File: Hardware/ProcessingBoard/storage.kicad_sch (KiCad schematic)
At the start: 21 parts, among them Q400 2N7002, U400 ADP163, U401 W25Q32JVZP

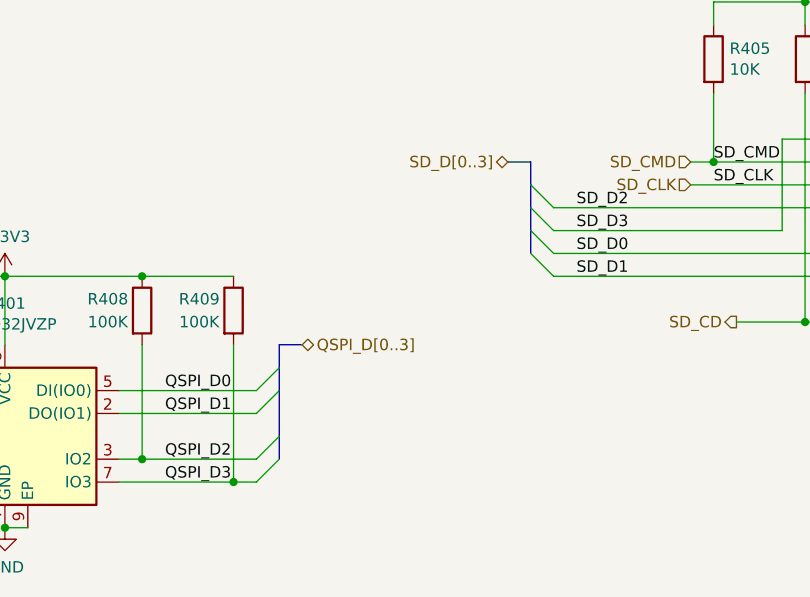
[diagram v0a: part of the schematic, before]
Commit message: Update License to match source code; test and fix USB, SEMC, and XIP on actual hardware
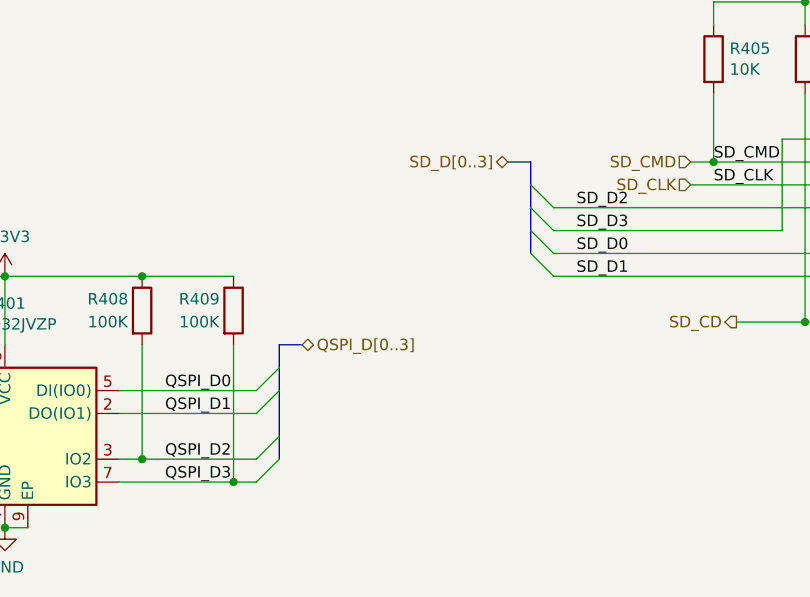
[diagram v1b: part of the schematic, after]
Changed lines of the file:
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@@
     (stroke (width 0) (type solid) (color 0 0 0 0))
   )
-  (bus (pts (xy 127 121.92) (xy 127 124.46))
+  (bus (pts (xy 127 121.92) (xy 127 134.62))
     (stroke (width 0) (type solid) (color 0 0 0 0))
   )
@@
     (stroke (width 0) (type solid) (color 0 0 0 0))
   )
-  (bus (pts (xy 127 124.46) (xy 127 127))
-    (stroke (width 0) (type solid) (color 0 0 0 0))
-  )
-  (bus (pts (xy 127 127) (xy 127 132.08))
-    (stroke (width 0) (type solid) (color 0 0 0 0))
-  )
-  (bus (pts (xy 127 132.08) (xy 127 134.62))
-    (stroke (width 0) (type solid) (color 0 0 0 0))
-  )
   (bus (pts (xy 154.94 101.6) (xy 152.4 101.6))
     (stroke (width 0) (type solid) (color 0 0 0 0))
   )
-  (bus (pts (xy 154.94 101.6) (xy 154.94 104.14))
+  (bus (pts (xy 154.94 101.6) (xy 154.94 111.76))
     (stroke (width 0) (type solid) (color 0 0 0 0))
   )
-  (bus (pts (xy 154.94 104.14) (xy 154.94 106.68))
-    (stroke (width 0) (type solid) (color 0 0 0 0))
-  )
-  (bus (pts (xy 154.94 106.68) (xy 154.94 109.22))
-    (stroke (width 0) (type solid) (color 0 0 0 0))
-  )
-  (bus (pts (xy 154.94 109.22) (xy 154.94 111.76))
-    (stroke (width 0) (type solid) (color 0 0 0 0))
-  )
